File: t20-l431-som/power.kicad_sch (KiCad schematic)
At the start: 42 parts, among them U1 STM32L431-WLCSP64, U2 T20W80, U4 MODULE_INTERNAL_T20_L431_HOST, U5 LP3986TL-2518/NOPB, U7 TPS22916BYFPR, U9 NCP139AFCT120T2G

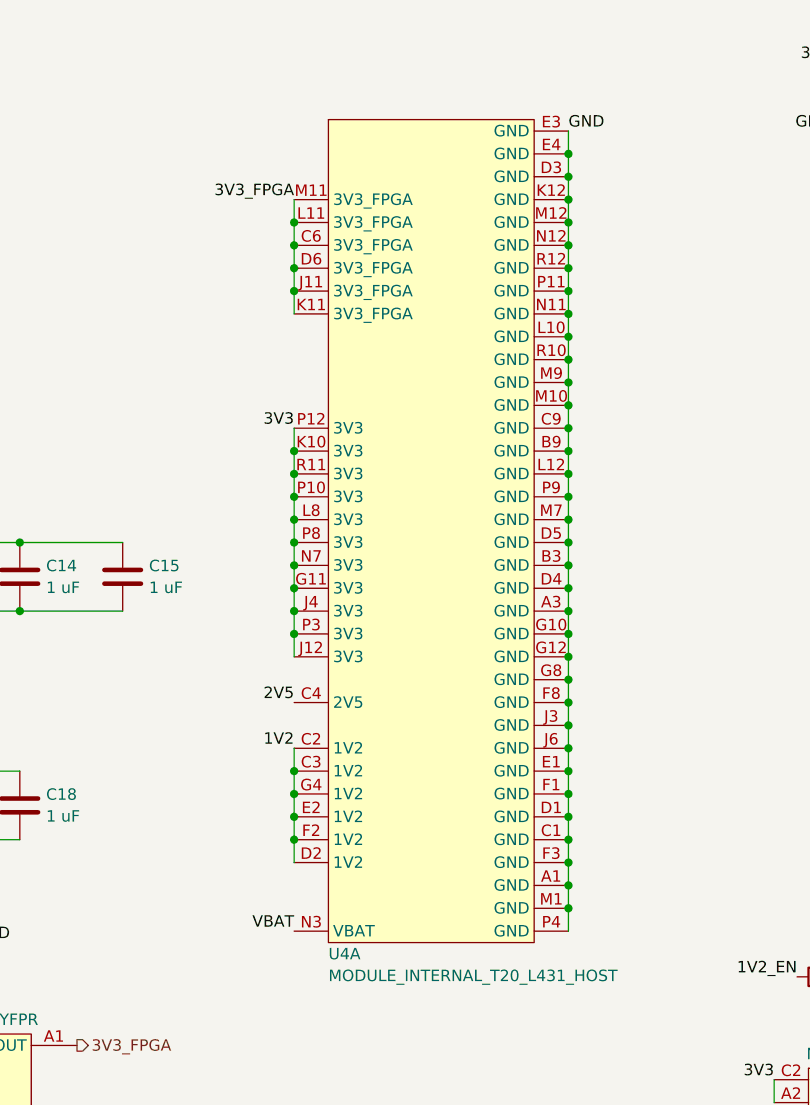
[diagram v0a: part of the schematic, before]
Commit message: Various layout fixes for DRC
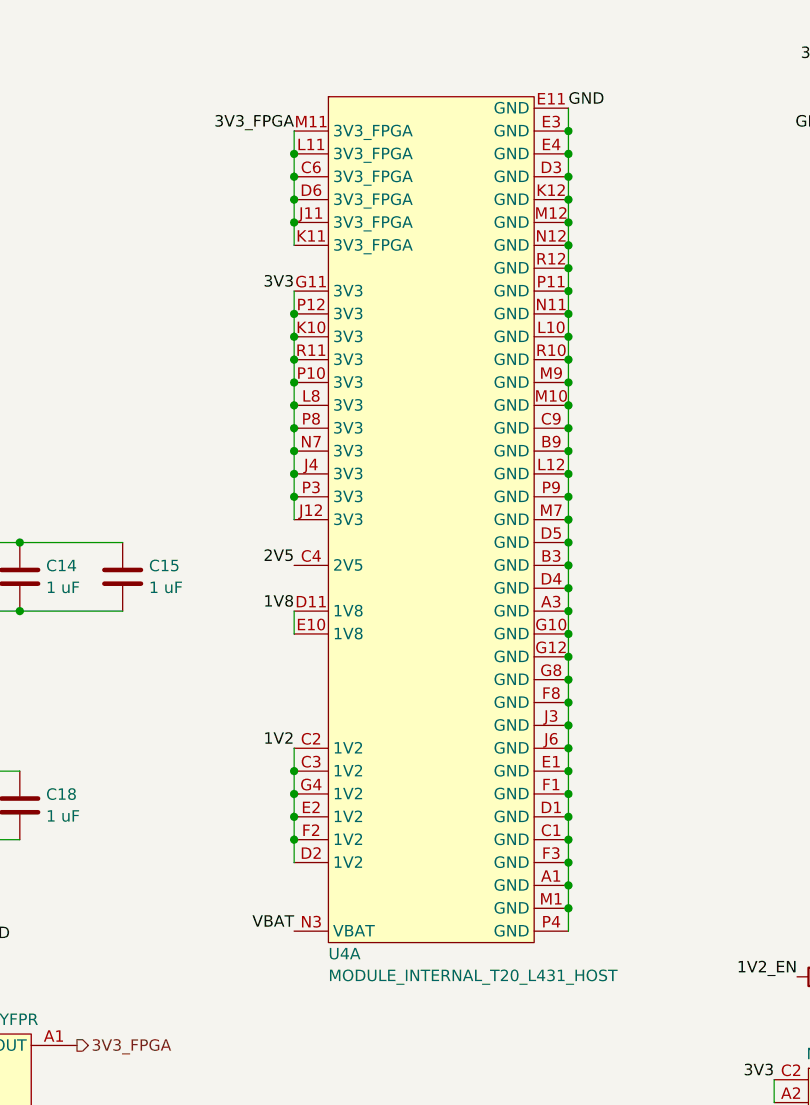
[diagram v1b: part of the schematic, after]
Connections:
- net 1V8: now also U4.D11 (1V8), U4.E10 (1V8)
- net GND: now also U4.E11 (GND)
